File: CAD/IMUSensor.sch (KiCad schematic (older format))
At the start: 5 parts, among them U6 LSM6DS33TR

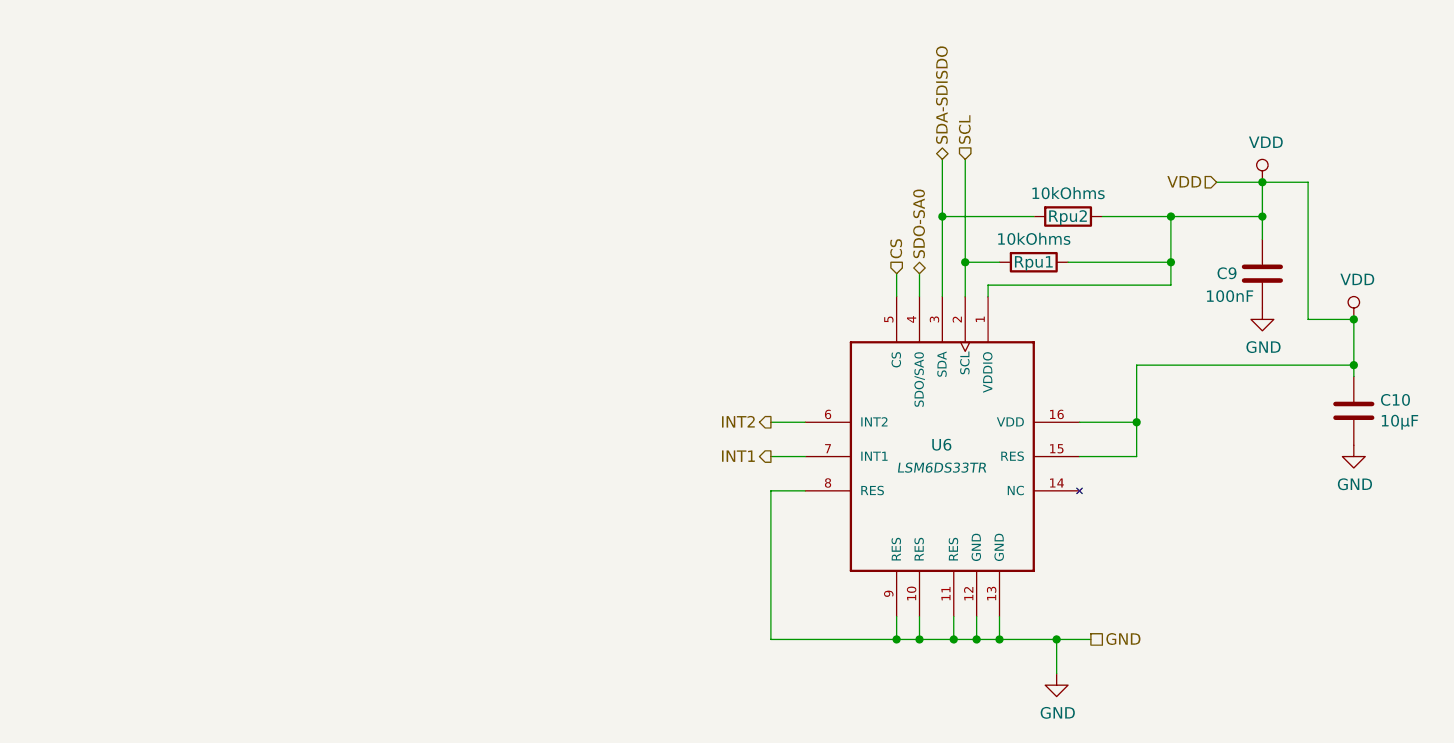
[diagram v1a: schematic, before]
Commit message: rescue commit
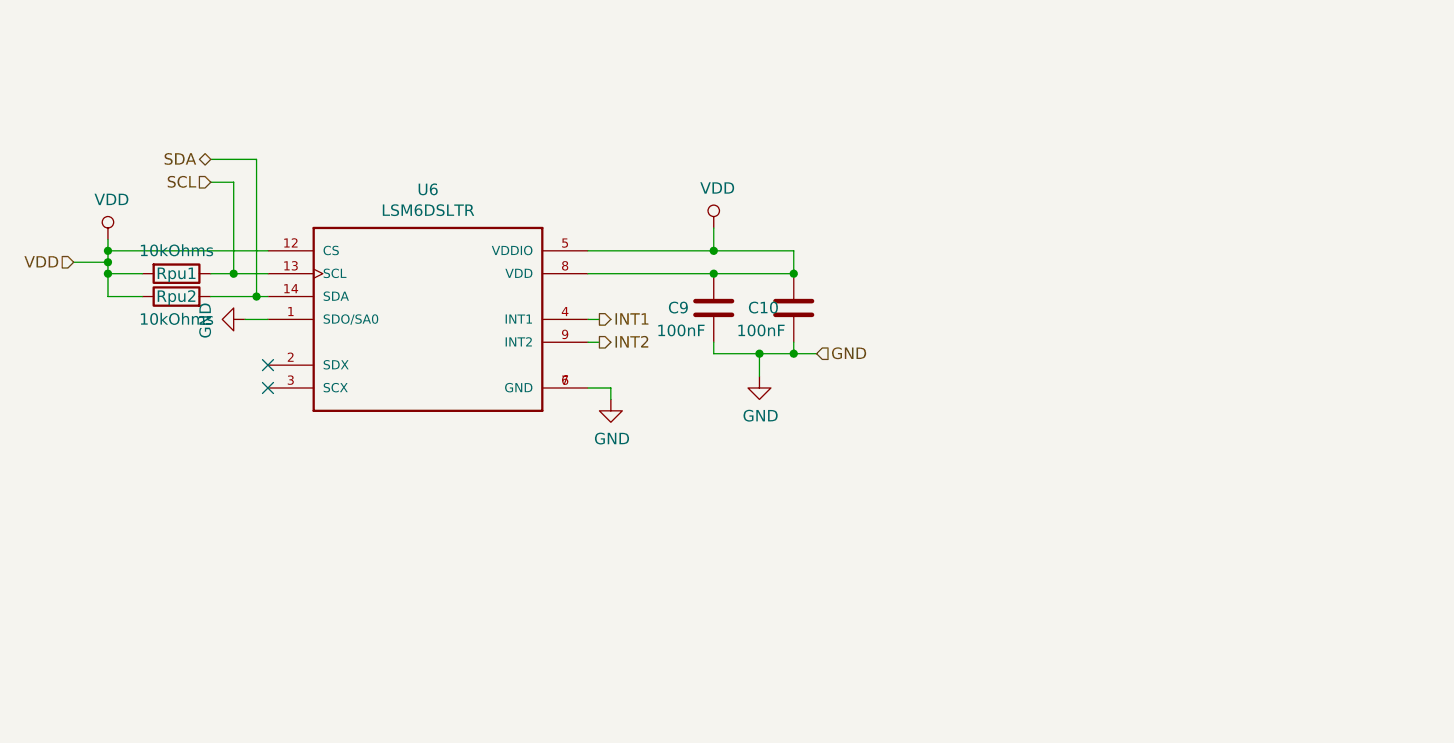
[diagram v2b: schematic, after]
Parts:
- removed U6: LSM6DS33TR, LSM6DS33TR:PQFN50P300X300X86-16N, symbol LSM6DS33TR:LSM6DS33TR
- added U6: LSM6DSLTR, LSM6DSLTR:PQFN50P300X250X86-14N, symbol LSM6DSLTR:LSM6DSLTR
- C10: value 10µF -> 100nF
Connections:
- net GND: now also U6.1 (SDO/SA0), U6.6 (GND), U6.7 (GND)
- net INT1: now also U6.4 (INT1)
- net INT2: now also U6.9 (INT2)
- net SCL: now also Rpu1.1, U6.13 (SCL); no longer Rpu1.2
- net VDD: now also Rpu1.2, U6.12 (CS), U6.5 (VDDIO), U6.8 (VDD); no longer Rpu1.1
- net SDA-SDISDO renamed SDA
- net SDA: now also U6.14 (SDA)
- no-connect marks 0 -> 2
